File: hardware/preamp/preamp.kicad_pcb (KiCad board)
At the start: 2 copper layers, 45 x 18 mm, 19 parts, among them J1 I/O, J4 Coil, U1 TLV170DBV

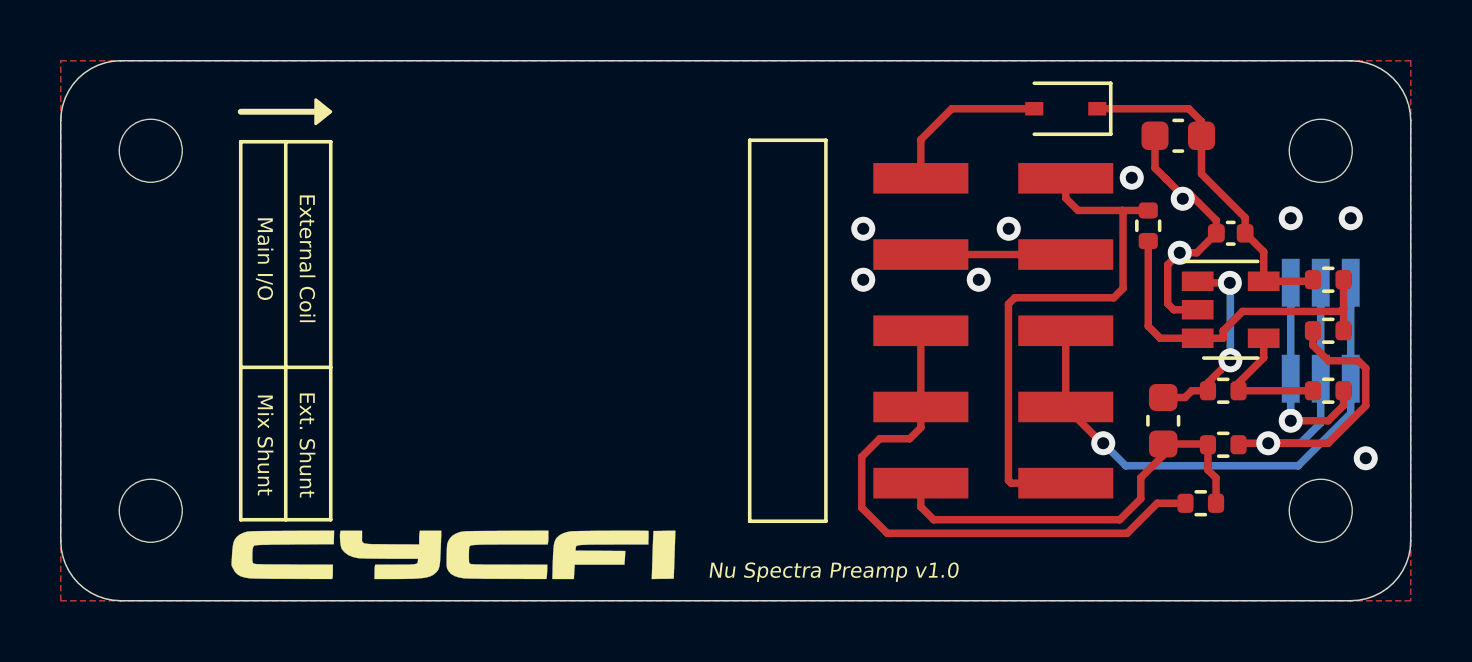
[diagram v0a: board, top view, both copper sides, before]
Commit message: Preamp updates
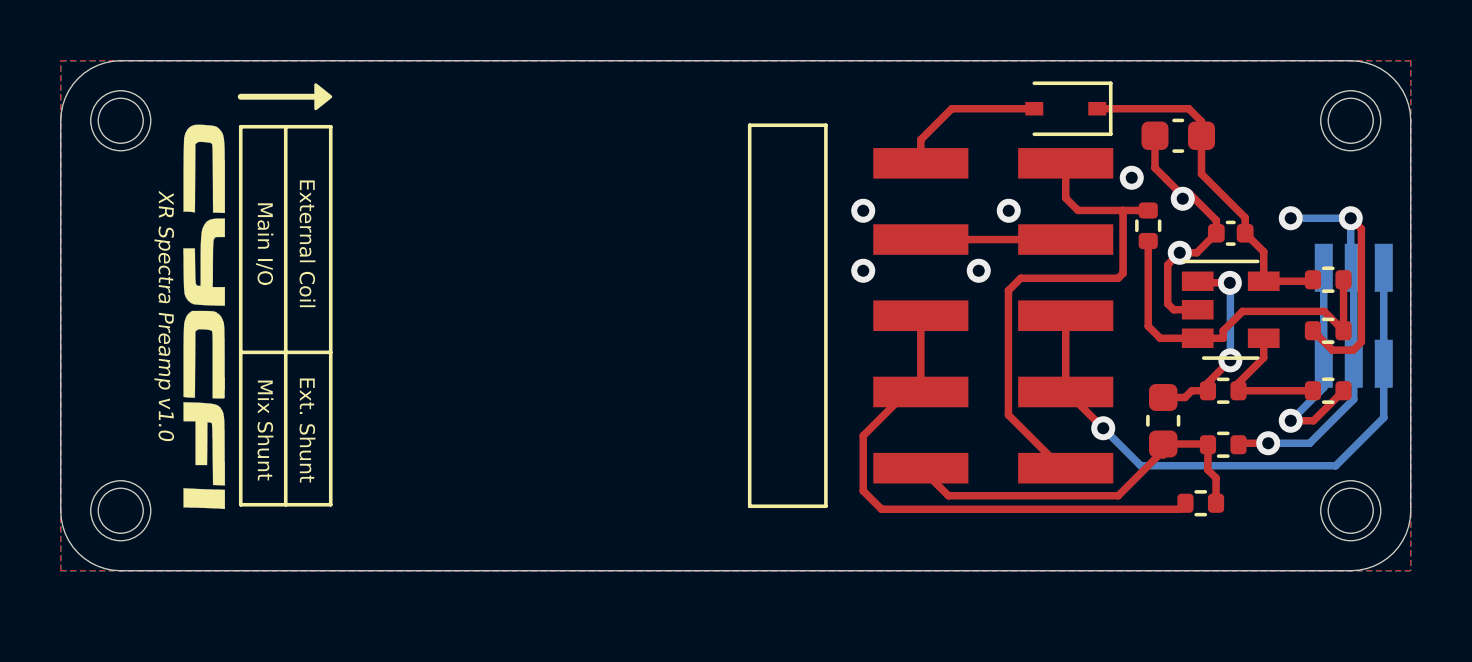
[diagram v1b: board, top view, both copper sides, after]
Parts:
- removed the G*** at (118.0, 116.5)
- added G***: LOGO, cycfi_library:cycfi-logo-12mm, F.Cu at (109.8, 108.5)
- H1, H2, H3, H4: footprint cycfi_library:mounting_hole_2.1mm -> cycfi_library:mounting_hole_st1.9
- moved H1 1.41 mm to (107.0, 102.0)
- moved H3 1.41 mm to (148.0, 102.0)
- moved J4 1.21 mm to (148.1, 108.5)
- moved H2 1.00 mm to (107.0, 115.0)
- moved H4 1.00 mm to (148.0, 115.0)
- moved J1 0.50 mm to (136.5, 108.5)
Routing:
- net GND: track 28.8 -> 32.7 mm, vias 11 -> 10
- net ext_coil+: track 18.1 -> 16.5 mm
- net out: track 14.3 -> 13.2 mm
- net ext_coil-: track 18.3 -> 19.3 mm
- net mix: track 18.9 -> 18.0 mm
- net /IN-: track 7.06 -> 7.73 mm
- net /VCC: track 5.50 -> 5.00 mm
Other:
- board size 45 x 18 mm -> 45 x 17 mm
- board text added: "XR Spectra Preamp v1.0"
- board text removed: "Nu Spectra Preamp v1.0"
